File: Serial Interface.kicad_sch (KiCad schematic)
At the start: 32 parts

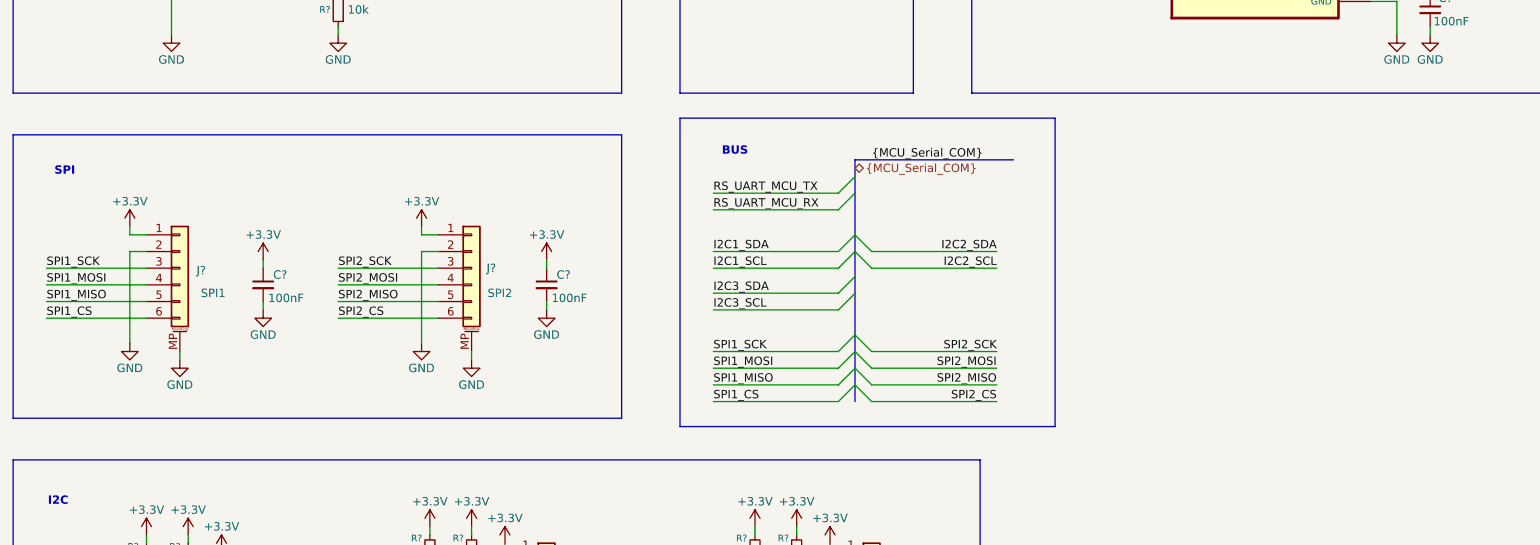
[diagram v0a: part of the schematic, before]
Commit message: IOT part Finilization
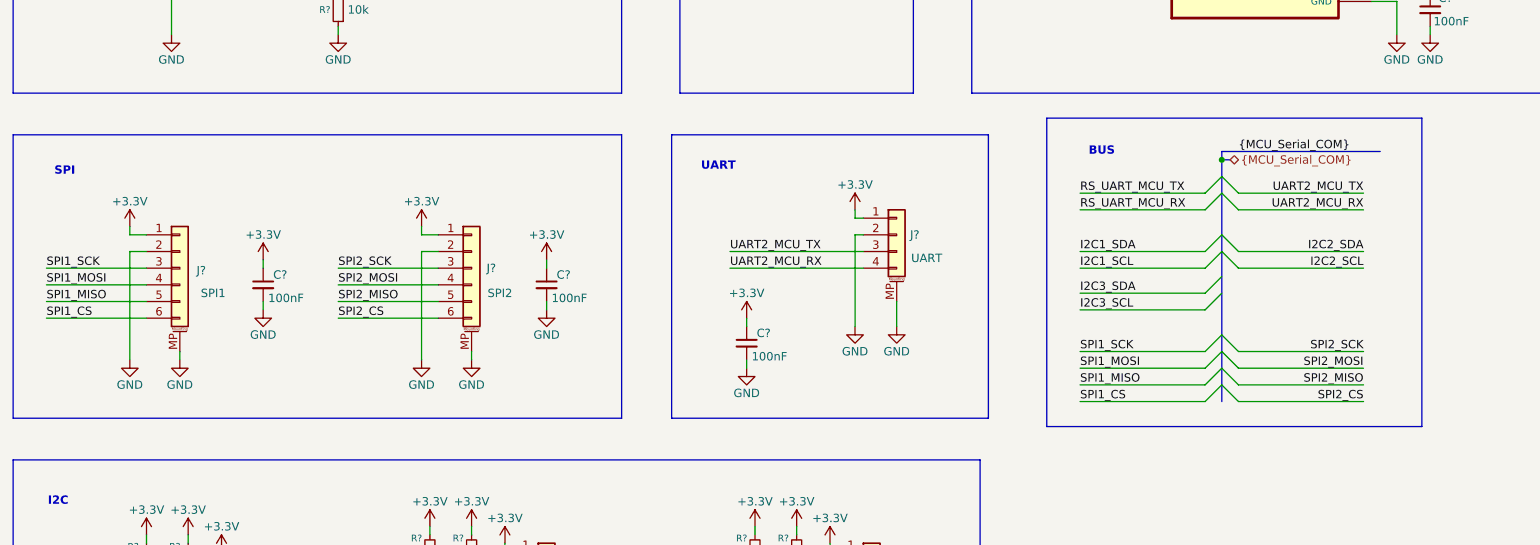
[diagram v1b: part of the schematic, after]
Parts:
- added C?: 100nF, Capacitor_SMD:C_0603_1608Metric_Pad1.08x0.95mm_HandSolder, symbol Device:C_Small
- added J?: *, Connector_JST:JST_PH_S4B-PH-SM4-TB_1x04-1MP_P2.00mm_Horizontal, symbol Connector_Generic_MountingPin:Conn_01x04_MountingPin
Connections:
- net +3.3V: now also C?.1, J?.1 (Pin_1)
- net GND: now also C?.2, J?.2 (Pin_2), J?.MP (MountPin)
- new net UART2_MCU_RX: J?.4 (Pin_4)
- new net UART2_MCU_TX: J?.3 (Pin_3)
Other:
- note added: "UART"
